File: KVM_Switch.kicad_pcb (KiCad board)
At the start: 6 copper layers, 120 x 120 mm, 77 parts, among them J1 USB_C_Host_B, J2 USB_C_Host_B, J3 Conn_01x02, SW1 SW_Push, U1 TLV62569DBV, U10 USB2514B_M2, U2 AP2112K-3.3, U3 STM32F030C8Tx, U4 TUSB1046A-DCIRNQR, U5 TUSB1046A-DCIRNQR, U6 HD3SS215RTQT, U9 TS3USB221RSERG4, Y1 Crystal

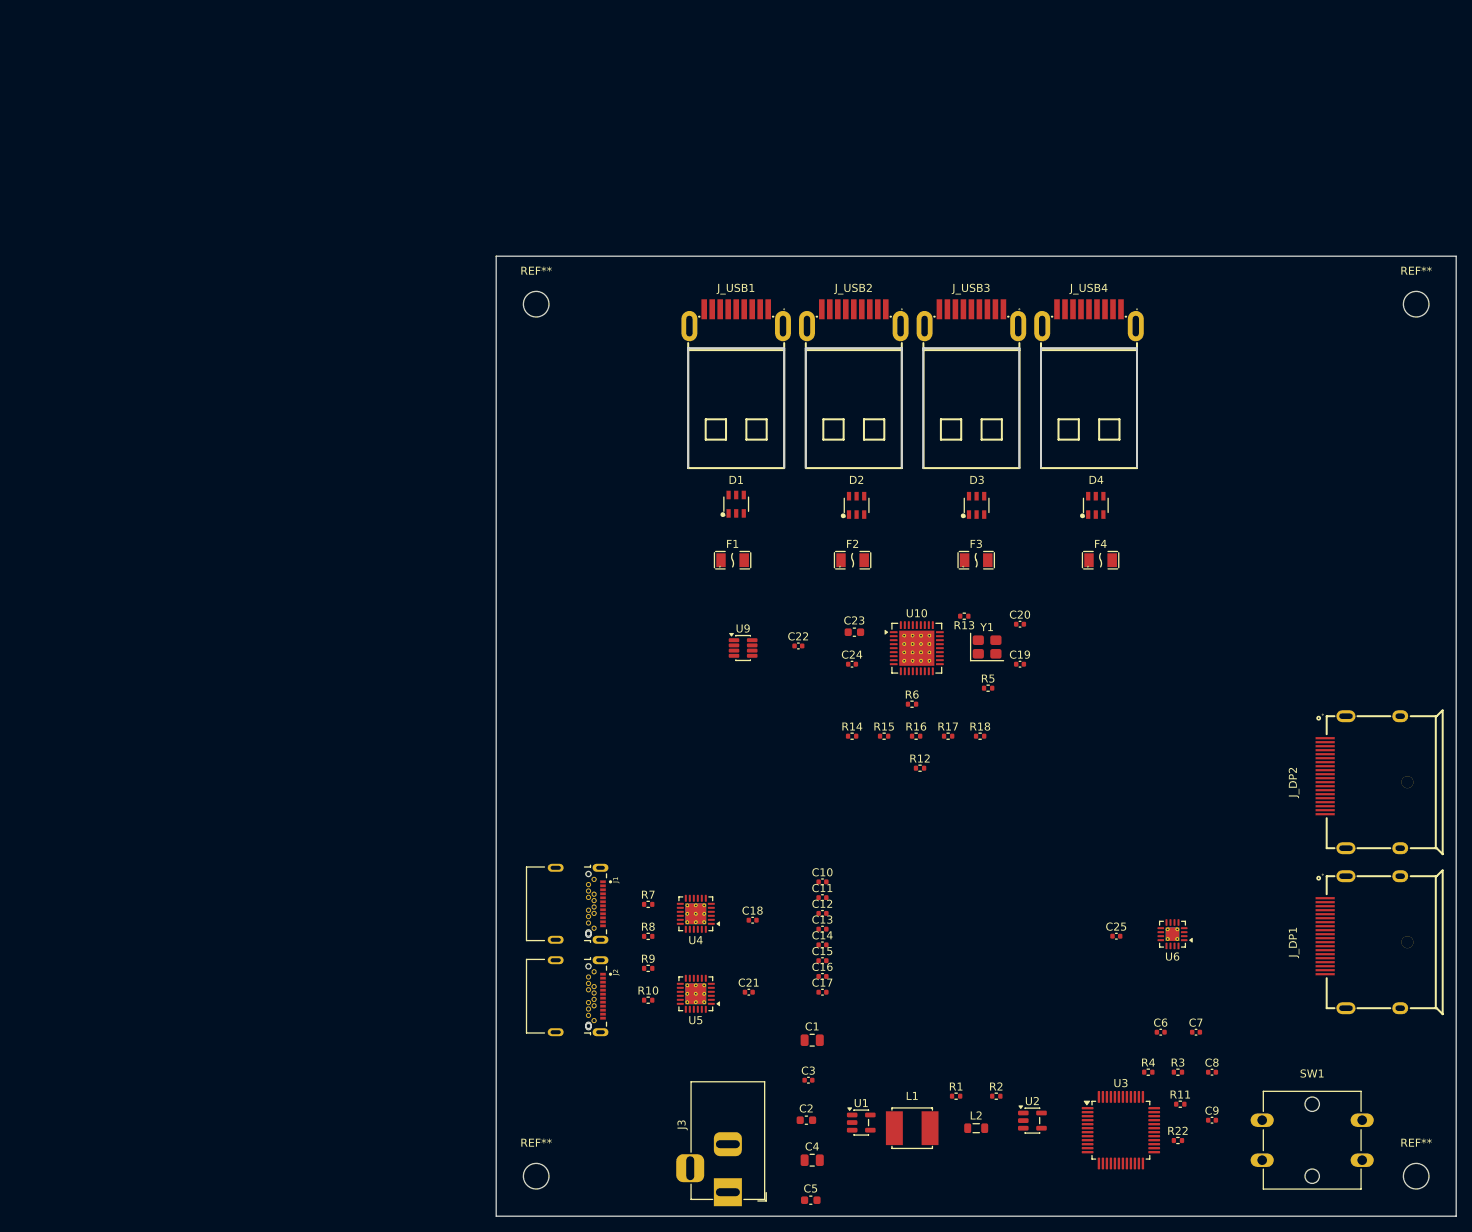
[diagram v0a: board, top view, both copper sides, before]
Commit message: Publish A2 hardware, firmware, and verification package
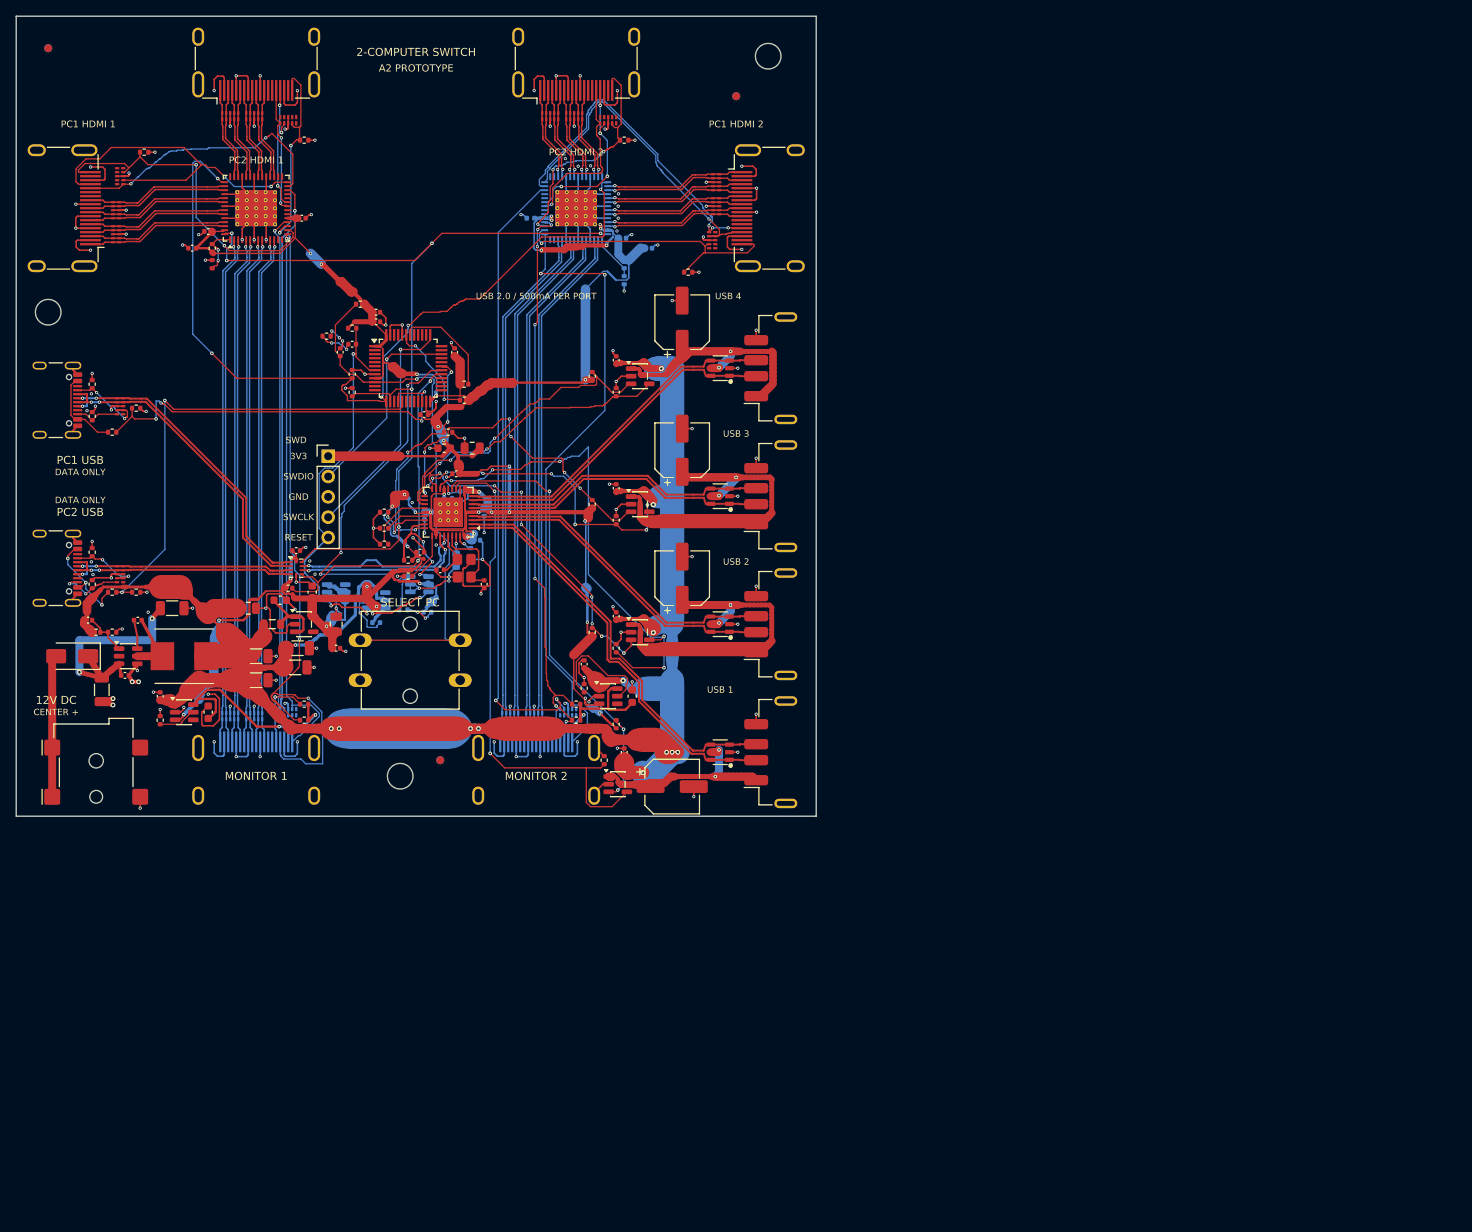
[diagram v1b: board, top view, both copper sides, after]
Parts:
- removed C17: 0.1uF, Capacitor_SMD:C_0402_1005Metric
- removed F1, F2, F3, F4: BSMD1206-050-6V, polyfuse:F1206
- removed J_DP1, J_DP2: 472720001, dp_connector:CONN-SMD_472720001
- removed R5: 1M, Resistor_SMD:R_0402_1005Metric
- removed REF** (x4): MountingHole_3.2mm_M3, MountingHole:MountingHole_3.2mm_M3
- added C26: 1uF, Capacitor_SMD:C_0603_1608Metric, F.Cu at (37.0, 72.0)
- added C27: 100nF, Capacitor_SMD:C_0402_1005Metric, F.Cu at (45.0, 38.2)
- added C28: 100nF, Capacitor_SMD:C_0402_1005Metric, F.Cu at (54.8, 42.0)
- added C29: 100nF, Capacitor_SMD:C_0402_1005Metric, F.Cu at (51.0, 49.8)
- added C30: 10uF, Capacitor_SMD:C_1206_3216Metric, F.Cu at (19.5, 74.0)
- added C31: 100nF, Capacitor_SMD:C_0402_1005Metric, F.Cu at (15.2, 75.5)
- added C32: 1uF, Capacitor_SMD:C_0603_1608Metric, F.Cu at (33.0, 73.0)
- added C33: 150pF, Capacitor_SMD:C_0402_1005Metric, F.Cu at (9.00, 75.5)
- added C34: 100nF, Capacitor_SMD:C_0402_1005Metric, F.Cu at (55.0, 57.2)
- added C35: 100nF, Capacitor_SMD:C_0402_1005Metric, B.Cu at (54.0, 60.3)
- added C36: 100nF, Capacitor_SMD:C_0402_1005Metric, B.Cu at (51.0, 62.4)
- added C37: 100nF, Capacitor_SMD:C_0402_1005Metric, F.Cu at (50.5, 67.0)
- added C38: 100nF, Capacitor_SMD:C_0402_1005Metric, B.Cu at (57.5, 65.5)
- added C39: 100nF, Capacitor_SMD:C_0402_1005Metric, F.Cu at (76.0, 92.0)
- added C40: 100nF, Capacitor_SMD:C_0402_1005Metric, F.Cu at (75.0, 75.0)
- added C41: 100nF, Capacitor_SMD:C_0402_1005Metric, F.Cu at (75.0, 59.0)
- added C42: 100nF, Capacitor_SMD:C_0402_1005Metric, F.Cu at (75.0, 43.0)
- added C43: 220uF, Capacitor_SMD:CP_Elec_6.3x7.7, F.Cu at (82.0, 96.3)
- added C44: 220uF, Capacitor_SMD:CP_Elec_6.3x7.7, F.Cu at (83.2, 70.2)
- added C45: 220uF, Capacitor_SMD:CP_Elec_6.3x7.7, F.Cu at (83.2, 54.2)
- added C46: 220uF, Capacitor_SMD:CP_Elec_6.3x7.7, F.Cu at (83.2, 38.2)
- added C47: 100nF, Capacitor_SMD:C_0402_1005Metric, F.Cu at (18.0, 85.0)
- added C48: 100nF, Capacitor_SMD:C_0402_1005Metric, F.Cu at (71.0, 81.0)
- added C49: 1uF, Capacitor_SMD:C_0603_1608Metric, F.Cu at (24.0, 87.0)
- added C50: 1uF, Capacitor_SMD:C_0603_1608Metric, F.Cu at (77.0, 85.0)
- added C51: 22uF, Capacitor_SMD:C_1206_3216Metric, F.Cu at (34.9, 81.4)
- added C52: 22uF, Capacitor_SMD:C_1206_3216Metric, F.Cu at (35.2, 79.0)
- added C53: 100nF, Capacitor_SMD:C_0402_1005Metric, B.Cu at (40.0, 74.8)
- added C54: 100nF, Capacitor_SMD:C_0402_1005Metric, B.Cu at (45.0, 75.8)
- added C55: 100nF, Capacitor_SMD:C_0402_1005Metric, B.Cu at (51.4, 74.5)
- added D20: SS34, Diode_SMD:D_SMA, F.Cu at (7.00, 80.0)
- added FID1: Fiducial_1mm_Mask2mm, Fiducial_1mm_Mask2mm, F.Cu at (4.00, 4.00)
- added FID2: Fiducial_1mm_Mask2mm, Fiducial_1mm_Mask2mm, F.Cu at (90.0, 10.0)
- added FID3: Fiducial_1mm_Mask2mm, Fiducial_1mm_Mask2mm, F.Cu at (53.0, 93.0)
- added FID4: Fiducial_1mm_Mask2mm, Fiducial_1mm_Mask2mm, B.Cu at (4.00, 4.00)
- added FID5: Fiducial_1mm_Mask2mm, Fiducial_1mm_Mask2mm, B.Cu at (90.0, 10.0)
- added FID6: Fiducial_1mm_Mask2mm, Fiducial_1mm_Mask2mm, B.Cu at (53.0, 93.0)
- added H1: M3 mounting, MountingHole_3.2mm_M3, F.Cu at (4.00, 37.0)
- added H2: M3 mounting, MountingHole_3.2mm_M3, F.Cu at (94.0, 5.00)
- added H3: M3 mounting, MountingHole_3.2mm_M3, F.Cu at (48.0, 95.0)
- added J4: SWD, Connector_PinHeader_2.54mm:PinHeader_1x05_P2.54mm_Vertical, F.Cu at (39.0, 55.0)
- added J_HDMI_C1_MON1: HDMI_A_1.4, KVM_Custom_Footprints:Assembly_J_HDMI_C1_MON1, F.Cu at (6.00, 24.0)
- added J_HDMI_C1_MON2: HDMI_A_1.4, KVM_Custom_Footprints:Assembly_J_HDMI_C1_MON2, F.Cu at (94.0, 24.0)
- added J_HDMI_C2_MON1: HDMI_A_1.4, KVM_Custom_Footprints:Assembly_J_HDMI_C2_MON1, F.Cu at (30.0, 6.00)
- added J_HDMI_C2_MON2: HDMI_A_1.4, KVM_Custom_Footprints:Assembly_J_HDMI_C2_MON2, F.Cu at (70.0, 6.00)
- added J_HDMI_MON1: HDMI_A_1.4, KVM_Custom_Footprints:Assembly_J_HDMI_MON1, B.Cu at (30.0, 94.0)
- added J_HDMI_MON2: HDMI_A_1.4, KVM_Custom_Footprints:Assembly_J_HDMI_MON2, B.Cu at (65.0, 94.0)
- added R19: 100k, Resistor_SMD:R_0402_1005Metric, F.Cu at (84.0, 32.0)
- added R20: 100k, Resistor_SMD:R_0402_1005Metric, F.Cu at (76.0, 15.5)
- added R23: 100k, Resistor_SMD:R_0402_1005Metric, F.Cu at (42.0, 47.0)
- added R24: 100k, Resistor_SMD:R_0402_1005Metric, F.Cu at (42.0, 44.8)
- added R25: 100k, Resistor_SMD:R_0402_1005Metric, F.Cu at (34.0, 71.5)
- added R26: 100k, Resistor_SMD:R_0402_1005Metric, F.Cu at (46.0, 64.0)
- added R27: 100k, Resistor_SMD:R_0402_1005Metric, F.Cu at (46.0, 62.0)
- added R28: 100k, Resistor_SMD:R_0402_1005Metric, F.Cu at (49.0, 70.0)
- added R29: 100k, Resistor_SMD:R_0402_1005Metric, F.Cu at (46.0, 66.0)
- added R30: 100k, Resistor_SMD:R_0402_1005Metric, F.Cu at (73.5, 93.0)
- added R31: 100k, Resistor_SMD:R_0402_1005Metric, F.Cu at (75.0, 79.0)
- added R32: 100k, Resistor_SMD:R_0402_1005Metric, F.Cu at (75.0, 63.0)
- added R33: 100k, Resistor_SMD:R_0402_1005Metric, F.Cu at (75.0, 47.0)
- added R34: 100k, Resistor_SMD:R_0402_1005Metric, F.Cu at (12.0, 52.0)
- added R35: 150k, Resistor_SMD:R_0402_1005Metric, F.Cu at (15.0, 49.0)
- added R36: 100k, Resistor_SMD:R_0402_1005Metric, F.Cu at (12.0, 72.0)
- added R37: 150k, Resistor_SMD:R_0402_1005Metric, F.Cu at (15.0, 72.0)
- added R38: 100k, Resistor_SMD:R_0402_1005Metric, F.Cu at (54.0, 52.0)
- added R39: 10k, Resistor_SMD:R_0402_1005Metric, F.Cu at (75.0, 88.5)
- added R40: 10k, Resistor_SMD:R_0402_1005Metric, F.Cu at (72.0, 77.0)
- added R41: 10k, Resistor_SMD:R_0402_1005Metric, F.Cu at (72.0, 61.0)
- added R42: 10k, Resistor_SMD:R_0402_1005Metric, F.Cu at (72.0, 45.0)
- added R43: 10k, Resistor_SMD:R_0402_1005Metric, F.Cu at (24.5, 29.0)
- added R44: 10k, KVM_Custom_Footprints:Assembly_R44, F.Cu at (24.5, 31.0)
- added R45: 10k, Resistor_SMD:R_0402_1005Metric, B.Cu at (76.0, 31.0)
- added R46: 10k, KVM_Custom_Footprints:Assembly_R46, B.Cu at (76.0, 33.0)
- added R47: 210k, Resistor_SMD:R_0402_1005Metric, F.Cu at (18.0, 88.0)
- added R48: 210k, Resistor_SMD:R_0402_1005Metric, F.Cu at (71.0, 84.0)
- added R49: 10k, Resistor_SMD:R_0402_1005Metric, B.Cu at (48.4, 74.2)
- added R50: 1k, Resistor_SMD:R_0402_1005Metric, F.Cu at (38.8, 40.0)
- added U11: TPD4E02B04DQA, KVM_Custom_Footprints:USON-10_2.5x1.0mm_P0.5mm_Assembly, B.Cu at (64.8, 87.5)
- added U12: TPD4E02B04DQA, KVM_Custom_Footprints:USON-10_2.5x1.0mm_P0.5mm_Assembly, F.Cu at (12.5, 27.2)
- added U13: TPD4E02B04DQA, KVM_Custom_Footprints:USON-10_2.5x1.0mm_P0.5mm_Assembly, F.Cu at (12.5, 24.2)
- added U14: TPD4E02B04DQA, KVM_Custom_Footprints:USON-10_2.5x1.0mm_P0.5mm_Assembly, F.Cu at (26.8, 12.5)
- added U15: TPD4E02B04DQA, KVM_Custom_Footprints:USON-10_2.5x1.0mm_P0.5mm_Assembly, F.Cu at (29.8, 12.5)
- added U16: TPD4E02B04DQA, KVM_Custom_Footprints:USON-10_2.5x1.0mm_P0.5mm_Assembly, F.Cu at (87.5, 20.8)
- added U17: TPD4E02B04DQA, KVM_Custom_Footprints:USON-10_2.5x1.0mm_P0.5mm_Assembly, F.Cu at (87.5, 23.8)
- added U18: TPD4E02B04DQA, KVM_Custom_Footprints:USON-10_2.5x1.0mm_P0.5mm_Assembly, F.Cu at (66.8, 12.5)
- added U19: TPD4E02B04DQA, KVM_Custom_Footprints:USON-10_2.5x1.0mm_P0.5mm_Assembly, F.Cu at (69.8, 12.5)
- added U20: TPS2051CDBVR, Package_TO_SOT_SMD:SOT-23-5, F.Cu at (75.2, 96.0)
- added U21: TPS2051CDBVR, Package_TO_SOT_SMD:SOT-23-5, F.Cu at (78.0, 77.0)
- added U22: TPS2051CDBVR, Package_TO_SOT_SMD:SOT-23-5, F.Cu at (78.0, 61.0)
- added U23: TPS2051CDBVR, Package_TO_SOT_SMD:SOT-23-5, F.Cu at (78.0, 45.0)
- added U24: TPD4E05U06DQAR, KVM_Custom_Footprints:USON-10_2.5x1.0mm_P0.5mm_Assembly, F.Cu at (13.0, 48.8)
- added U25: TPD4E05U06DQAR, KVM_Custom_Footprints:USON-10_2.5x1.0mm_P0.5mm_Assembly, F.Cu at (13.0, 69.8)
- added U26: TPD4E05U06DQAR, KVM_Custom_Footprints:USON-10_2.5x1.0mm_P0.5mm_Assembly, F.Cu at (13.0, 20.0)
- added U27: TPD4E05U06DQAR, KVM_Custom_Footprints:USON-10_2.5x1.0mm_P0.5mm_Assembly, F.Cu at (34.0, 13.0)
- added U28: TPD4E05U06DQAR, KVM_Custom_Footprints:USON-10_2.5x1.0mm_P0.5mm_Assembly, F.Cu at (87.0, 28.0)
- added U29: TPD4E05U06DQAR, KVM_Custom_Footprints:USON-10_2.5x1.0mm_P0.5mm_Assembly, F.Cu at (74.0, 13.0)
- added U30: TPD4E05U06DQAR, KVM_Custom_Footprints:USON-10_2.5x1.0mm_P0.5mm_Assembly, B.Cu at (34.0, 87.0)
- added U31: TPD4E05U06DQAR, KVM_Custom_Footprints:USON-10_2.5x1.0mm_P0.5mm_Assembly, B.Cu at (69.0, 87.0)
- added U32: TPS2553DBVR, Package_TO_SOT_SMD:SOT-23-6, F.Cu at (21.0, 87.0)
- added U33: TPS2553DBVR, Package_TO_SOT_SMD:SOT-23-6, F.Cu at (74.0, 85.0)
- added U34: TPS3808G33DBVR, Package_TO_SOT_SMD:SOT-23-6, B.Cu at (40.0, 72.0)
- added U35: TPS3808G50DBVR, Package_TO_SOT_SMD:SOT-23-6, B.Cu at (45.0, 73.0)
- added U36: SN74LVC1G97DBVR, Package_TO_SOT_SMD:SOT-23-6, B.Cu at (50.4, 71.0)
- added U7: TPD4E02B04DQA, KVM_Custom_Footprints:USON-10_2.5x1.0mm_P0.5mm_Assembly, B.Cu at (61.8, 87.5)
- added U8: HD3SS215IRTQR, Package_DFN_QFN:QFN-56-1EP_8x8mm_P0.5mm_EP4.5x5.2mm_ThermalVias, B.Cu at (70.0, 24.0)
- C1, C4: value 47uF -> 22uF; footprint Capacitor_SMD:C_0805_2012Metric -> Capacitor_SMD:C_1206_3216Metric
- C13, C14, C15, R12: moved to B.Cu
- C16: value 0.1uF -> 10uF; footprint Capacitor_SMD:C_0402_1005Metric -> Capacitor_SMD:C_1206_3216Metric
- C18: value 1uF -> 100nF; footprint Capacitor_SMD:C_0402_1005Metric -> Capacitor_SMD:C_0603_1608Metric; moved to B.Cu
- C19, C20: value 22pF -> 18pF
- C2, C23, C5: footprint Capacitor_SMD:C_0603_1608Metric -> Capacitor_SMD:C_0805_2012Metric
- C21: value 1uF -> 100nF; moved to B.Cu
- C22: value 0.1uF -> 100nF; moved to B.Cu
- C24: footprint Capacitor_SMD:C_0402_1005Metric -> Capacitor_SMD:C_0603_1608Metric
- C25: value 0.1uF -> 100nF
- J1, J2: value USB_C_Host_B -> USB4105-GF-A-120; footprint KVM_Custom_Footprints:CUI_UJ31-CH-G2-SMT-TR -> Connector_USB:USB_C_Receptacle_GCT_USB4105-xx-A_16P_TopMnt_Horizontal
- J3: value Conn_01x02 -> 12V DC center-positive; footprint Connector_BarrelJack:BarrelJack_Horizontal -> Connector_BarrelJack:BarrelJack_Wuerth_694106106102_2.0x5.5mm
- J_USB1: value KH-3.0USB-AM-9P -> USB1046-GF-0190-L-B-A; footprint usb_a_connector:USB-3.0-SMD_KH-3.0USB-AM-9P -> KVM_Custom_Footprints:Assembly_J_USB1
- J_USB2: value KH-3.0USB-AM-9P -> USB1046-GF-0190-L-B-A; footprint usb_a_connector:USB-3.0-SMD_KH-3.0USB-AM-9P -> KVM_Custom_Footprints:Assembly_J_USB2
- J_USB3: value KH-3.0USB-AM-9P -> USB1046-GF-0190-L-B-A; footprint usb_a_connector:USB-3.0-SMD_KH-3.0USB-AM-9P -> KVM_Custom_Footprints:Assembly_J_USB3
- J_USB4: value KH-3.0USB-AM-9P -> USB1046-GF-0190-L-B-A; footprint usb_a_connector:USB-3.0-SMD_KH-3.0USB-AM-9P -> KVM_Custom_Footprints:Assembly_J_USB4
- L1: value 4.7uH -> 6.8uH; footprint inductor_5040:IND-SMD_L5.0-W5.0-1 -> KVM_Custom_Footprints:Bourns_SRP7050TA
- R1: value 750k -> 53.6k
- R14, R15, R16, R6: value 100k -> 47k
- R2: value 100k -> 10k
- U1: value TLV62569DBV -> AP63301WU-7; footprint Package_TO_SOT_SMD:SOT-23-5 -> Package_TO_SOT_SMD:SOT-23-6
- U10: value USB2514B_M2 -> USB2514B-AEZC-TR; footprint Package_DFN_QFN:Texas_RHH0036C_VQFN-36-1EP_6x6mm_P0.5mm_EP4.4x4.4mm_ThermalVias -> Package_DFN_QFN:QFN-36-1EP_6x6mm_P0.5mm_EP3.7x3.7mm_ThermalVias
- U2: value AP2112K-3.3 -> AP2112K-3.3TRG1
- U4, U5: value TUSB1046A-DCIRNQR -> TPD4E02B04DQA; footprint Package_DFN_QFN:WQFN-24-1EP_4x4mm_P0.5mm_EP2.6x2.6mm_ThermalVias -> KVM_Custom_Footprints:USON-10_2.5x1.0mm_P0.5mm_Assembly; moved to B.Cu
- U6: value HD3SS215RTQT -> HD3SS215IRTQR; footprint Package_DFN_QFN:QFN-16-1EP_3x3mm_P0.5mm_EP1.7x1.7mm_ThermalVias -> Package_DFN_QFN:QFN-56-1EP_8x8mm_P0.5mm_EP4.5x5.2mm_ThermalVias
- U9: value TS3USB221RSERG4 -> TS3USB221RSER; footprint Package_TO_SOT_SMD:SOT-23-8 -> Package_DFN_QFN:Texas_UQFN-10_1.5x2mm_P0.5mm
- Y1: value Crystal -> 24MHz 12pF; footprint Crystal:Crystal_SMD_3225-4Pin_3.2x2.5mm -> KVM_Custom_Footprints:Assembly_Y1
- moved U6 146.1 mm to (30.0, 24.0), turned to 90 degrees
- moved C9 145.2 mm to (40.5, 42.0), turned to 90 degrees
- moved C8 140.8 mm to (42.0, 41.0)
- moved R3 138.9 mm to (42.0, 39.0)
- moved R4 137.6 mm to (43.0, 36.0)
- moved C6 133.1 mm to (45.0, 37.0)
- moved U3 130.4 mm to (49.0, 44.0)
- moved R22 128.5 mm to (56.0, 48.0)
- moved SW1 127.7 mm to (43.0, 78.0)
- moved R11 126.9 mm to (56.0, 46.0)
- moved R2 124.8 mm to (12.0, 77.0)
- moved R17 124.2 mm to (16.0, 17.0)
- moved R1 122.1 mm to (10.0, 77.0)
- moved C7 117.7 mm to (40.0, 79.0)
- moved C25 113.3 mm to (35.0, 66.8)
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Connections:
- net Net-(J1-CC1) renamed HOST1_CC1
- net Net-(J1-CC2) renamed HOST1_CC2
- net Net-(J2-CC1) renamed HOST2_CC1
- net Net-(J2-CC2) renamed HOST2_CC2
- net Net-(U10-DM-UP) renamed USB_UP_N
- net Net-(U10-DP-UP) renamed USB_UP_P
- net Net-(U10-~{RESET}) renamed HUB_RESET_N
- net Net-(U2-EN) renamed LDO_VIN
- net Net-(U3-NRST) renamed MCU_NRST
- net USB2_DN_A renamed USB_HOST1_N
- net USB2_DN_B renamed USB_HOST2_N
- net USB2_DP_A renamed USB_HOST1_P
- net USB2_DP_B renamed USB_HOST2_P
- C10 pad 1: Net-(U4-TX2P) -> +3.3V
- C10 pad 2: Net-(U6-DC0(p)) -> GND
- C11 pad 1: Net-(U6-DC0(n)) -> +3.3V
- C11 pad 2: Net-(U4-TX2N) -> GND
- C12 pad 1: Net-(U6-DC2(n)) -> +3.3V
- C12 pad 2: Net-(U4-TX1N) -> GND
- C13 pad 1: Net-(U6-DC2(p)) -> +3.3V
- C13 pad 2: Net-(U4-TX1P) -> GND
- C14 pad 1: Net-(U5-TX2P) -> +3.3V
- C14 pad 2: Net-(U6-DC1(p)) -> GND
- C15 pad 1: Net-(U6-DC1(n)) -> +3.3V
- C15 pad 2: Net-(U5-TX2N) -> GND
- C16 pad 1: Net-(U5-TX1P) -> +VIN
- C16 pad 2: Net-(U6-DC3(p)) -> GND
- C18 pad 1: GND -> HUB_PLLFILT
- C18 pad 2: Net-(U10-PLLFILT) -> GND
- C19 pad 1: GND -> HUB_XTAL1
- C19 pad 2: Net-(U10-XTAL1) -> GND
- C20 pad 1: Net-(U10-XTAL2) -> HUB_XTAL2
- C21 pad 1: GND -> HUB_CRFILT
- C21 pad 2: Net-(U10-CRFILT) -> GND
- C22 pad 1: GND -> +3.3V
- C22 pad 2: +3.3V -> GND
- C23 pad 1: GND -> +3.3V
- C23 pad 2: +3.3V -> GND
- C24 pad 1: GND -> +3.3V
- C24 pad 2: +3.3V -> GND
- C25 pad 1: Net-(U9-VCC) -> +3.3V
- C25 pad 2: +3.3V -> GND
- C3 pad 1: +5V -> +VIN
- C8 pad 1: GND -> RESET_CAP_RETURN
- D1 pad 1: /USB_Hub_ESD/USB_D1_N -> USB_D1_N
- D1 pad 3: /USB_Hub_ESD/USB_D1_P -> USB_D1_P
- D1 pad 4: /USB_Hub_ESD/USB1_DP -> USB_D1_P
- D1 pad 5: +5V -> USB_VBUS1
- D1 pad 6: /USB_Hub_ESD/USB1_DM -> USB_D1_N
- D2 pad 1: /USB_Hub_ESD/USB_D2_N -> USB_D2_N
- D2 pad 3: /USB_Hub_ESD/USB_D2_P -> USB_D2_P
- D2 pad 4: /USB_Hub_ESD/USB2_DP -> USB_D2_P
- D2 pad 5: +5V -> USB_VBUS2
- D2 pad 6: /USB_Hub_ESD/USB2_DM -> USB_D2_N
- D3 pad 1: /USB_Hub_ESD/USB_D3_N -> USB_D3_N
- D3 pad 3: /USB_Hub_ESD/USB_D3_P -> USB_D3_P
- D3 pad 4: /USB_Hub_ESD/USB3_DP -> USB_D3_P
- D3 pad 5: +5V -> USB_VBUS3
- D3 pad 6: /USB_Hub_ESD/USB3_DM -> USB_D3_N
- D4 pad 1: /USB_Hub_ESD/USB_D4_N -> USB_D4_N
- D4 pad 3: /USB_Hub_ESD/USB_D4_P -> USB_D4_P
- D4 pad 4: /USB_Hub_ESD/USB4_DP -> USB_D4_P
- D4 pad 5: +5V -> USB_VBUS4
- D4 pad 6: /USB_Hub_ESD/USB4_DM -> USB_D4_N
- J1 pad A4: unconnected-(J1-VBUS-PadA4)_2 -> HOST1_VBUS
- J1 pad A8: Net-(J1-SBU1) -> unconnected-(J1-SBU1-PadA8)
- J1 pad A9: unconnected-(J1-VBUS-PadA4)_1 -> HOST1_VBUS
- J1 pad B4: unconnected-(J1-VBUS-PadA4) -> HOST1_VBUS
- J1 pad B8: Net-(J1-SBU2) -> unconnected-(J1-SBU2-PadB8)
- J1 pad B9: unconnected-(J1-VBUS-PadA4)_3 -> HOST1_VBUS
- J2 pad A4: unconnected-(J2-VBUS-PadA4)_3 -> HOST2_VBUS
- J2 pad A8: Net-(J2-SBU1) -> unconnected-(J2-SBU1-PadA8)
- J2 pad A9: unconnected-(J2-VBUS-PadA4)_2 -> HOST2_VBUS
- J2 pad B4: unconnected-(J2-VBUS-PadA4) -> HOST2_VBUS
- J2 pad B8: Net-(J2-SBU2) -> unconnected-(J2-SBU2-PadB8)
- J2 pad B9: unconnected-(J2-VBUS-PadA4)_1 -> HOST2_VBUS
- J3 pad 1: /PDN/+VIN -> VIN_RAW
- J_USB1 pad 1: /USB_Hub_ESD/USB1_VBUS -> USB_VBUS1
- J_USB1 pad 2: /USB_Hub_ESD/USB1_DM -> USB_D1_N
- J_USB1 pad 3: /USB_Hub_ESD/USB1_DP -> USB_D1_P
- J_USB2 pad 1: /USB_Hub_ESD/USB2_VBUS -> USB_VBUS2
- J_USB2 pad 2: /USB_Hub_ESD/USB2_DM -> USB_D2_N
- J_USB2 pad 3: /USB_Hub_ESD/USB2_DP -> USB_D2_P
- J_USB3 pad 1: /USB_Hub_ESD/USB3_VBUS -> USB_VBUS3
- J_USB3 pad 2: /USB_Hub_ESD/USB3_DM -> USB_D3_N
- J_USB3 pad 3: /USB_Hub_ESD/USB3_DP -> USB_D3_P
- J_USB4 pad 1: /USB_Hub_ESD/USB4_VBUS -> USB_VBUS4
- J_USB4 pad 2: /USB_Hub_ESD/USB4_DM -> USB_D4_N
- J_USB4 pad 3: /USB_Hub_ESD/USB4_DP -> USB_D4_P
- L1 pad 1: Net-(U1-SW) -> BUCK_SW
- R1 pad 1: Net-(U1-FB) -> +5V
- R1 pad 2: +5V -> BUCK_FB
- R12 pad 1: GND -> HUB_RBIAS
- R12 pad 2: Net-(U10-RBIAS) -> GND
- R14 pad 1: GND -> /USBC_Mux/MON1_DDC_DAT
- R14 pad 2: Net-(J_DP1-Pad14) -> HDMI_MON1_5V
- R15 pad 1: /USBC_Mux/HPDA -> /USBC_Mux/MON2_DDC_CLK
- R15 pad 2: GND -> HDMI_MON2_5V
- R16 pad 1: GND -> /USBC_Mux/MON2_DDC_DAT
- R16 pad 2: Net-(J_DP2-Pad14) -> HDMI_MON2_5V
- R17 pad 1: /USBC_Mux/HPDB -> /USBC_Mux/C1_MON1_HPD
- R18 pad 1: GND -> /USBC_Mux/C2_MON1_HPD
- R18 pad 2: Net-(J_DP2-Pad13) -> GND
- R2 pad 1: Net-(U1-FB) -> BUCK_FB
- R6 pad 1: GND -> /USBC_Mux/MON1_DDC_CLK
- R6 pad 2: Net-(J_DP1-Pad13) -> HDMI_MON1_5V
- U1 pad 1: /PDN/+VIN -> BUCK_FB
- U1 pad 2: GND -> unconnected-(U1-EN-Pad2)
- U1 pad 3: Net-(U1-SW) -> +VIN
- U1 pad 4: /PDN/+VIN -> GND
- U1 pad 5: Net-(U1-FB) -> BUCK_SW
- U10 pad 1: /USB_Hub_ESD/USB_D1_N -> USB_D1_N
- U10 pad 12: unconnected-(U10-PRTPWR1-Pad12) -> USB_PWR1
- U10 pad 13: unconnected-(U10-OCS1-Pad13) -> USB_OC1_N
- U10 pad 14: Net-(U10-CRFILT) -> HUB_CRFILT
- U10 pad 16: unconnected-(U10-PRTPWR2-Pad16) -> USB_PWR2
- U10 pad 17: unconnected-(U10-OCS2-Pad17) -> USB_OC2_N
- U10 pad 18: unconnected-(U10-PRTPWR3-Pad18) -> USB_PWR3
- U10 pad 19: unconnected-(U10-OCS3-Pad19) -> USB_OC3_N
- U10 pad 2: /USB_Hub_ESD/USB_D1_P -> USB_D1_P
- U10 pad 20: unconnected-(U10-PRTPWR4-Pad20) -> USB_PWR4
- U10 pad 21: unconnected-(U10-OCS4-Pad21) -> USB_OC4_N
- U10 pad 22: unconnected-(U10-SMBDATA-Pad22) -> HUB_NONREM1
- U10 pad 24: unconnected-(U10-SMBCLK-Pad24) -> HUB_CFG0
- U10 pad 25: GND -> HUB_CFG1
- U10 pad 27: +3.3V -> HUB_VBUS_DET
- U10 pad 28: unconnected-(U10-SUSP_IND-Pad28) -> HUB_NONREM0
- U10 pad 3: /USB_Hub_ESD/USB_D2_N -> USB_D2_N
- U10 pad 32: Net-(U10-XTAL1) -> HUB_XTAL1
- U10 pad 33: Net-(U10-XTAL2) -> HUB_XTAL2
- U10 pad 34: Net-(U10-PLLFILT) -> HUB_PLLFILT
- U10 pad 35: Net-(U10-RBIAS) -> HUB_RBIAS
- U10 pad 4: /USB_Hub_ESD/USB_D2_P -> USB_D2_P
- U10 pad 6: /USB_Hub_ESD/USB_D3_N -> USB_D3_N
- U10 pad 7: /USB_Hub_ESD/USB_D3_P -> USB_D3_P
- U10 pad 8: /USB_Hub_ESD/USB_D4_N -> USB_D4_N
- U10 pad 9: /USB_Hub_ESD/USB_D4_P -> USB_D4_P
- U3 pad 11: TUSB2_SEL -> unconnected-(U3-PA1-Pad11)
- U3 pad 12: TUSB1_SEL -> unconnected-(U3-PA2-Pad12)
- U3 pad 16: unconnected-(U3-PA6-Pad16) -> HOST1_PRESENT
- U3 pad 17: unconnected-(U3-PA7-Pad17) -> HOST2_PRESENT
- U3 pad 29: unconnected-(U3-PA8-Pad29) -> USB_OE_N
- U3 pad 30: unconnected-(U3-PA9-Pad30) -> HUB_RESET_REQ
- U3 pad 31: unconnected-(U3-PA10-Pad31) -> HUB_VBUS_DET
- U3 pad 34: unconnected-(U3-PA13-Pad34) -> SWDIO
- U3 pad 37: unconnected-(U3-PA14-Pad37) -> SWCLK
- U4 pad 1: +3.3V -> /USBC_Mux/MON1_D2_P
- U4 pad 10: Net-(J1-TX2+) -> /USBC_Mux/MON1_D2_P
- U4 pad 2: unconnected-(U4-DPEQ1-Pad2) -> /USBC_Mux/MON1_D2_N
- U4 pad 3: unconnected-(U4-SSEQ1-Pad3) -> GND
- U4 pad 4: Net-(J1-TX1+) -> /USBC_Mux/MON1_D1_P
- U4 pad 5: Net-(J1-TX1-) -> /USBC_Mux/MON1_D1_N
- U4 pad 6: +3.3V -> /USBC_Mux/MON1_D1_N
- U4 pad 7: Net-(J1-RX1+) -> /USBC_Mux/MON1_D1_P
- U4 pad 8: Net-(J1-RX1-) -> GND
- U4 pad 9: Net-(J1-TX2-) -> /USBC_Mux/MON1_D2_N
- U5 pad 1: +3.3V -> /USBC_Mux/MON1_D0_P
- U5 pad 10: Net-(J2-TX2+) -> /USBC_Mux/MON1_D0_P
- U5 pad 2: unconnected-(U5-DPEQ1-Pad2) -> /USBC_Mux/MON1_D0_N
- U5 pad 3: unconnected-(U5-SSEQ1-Pad3) -> GND
- U5 pad 4: Net-(J2-TX1+) -> /USBC_Mux/MON1_D3_P
- U5 pad 5: Net-(J2-TX1-) -> /USBC_Mux/MON1_D3_N
- U5 pad 6: +3.3V -> /USBC_Mux/MON1_D3_N
- U5 pad 7: Net-(J2-RX1+) -> /USBC_Mux/MON1_D3_P
- U5 pad 8: Net-(J2-RX1-) -> GND
- U5 pad 9: Net-(J2-TX2-) -> /USBC_Mux/MON1_D0_N
- U6 pad 1: unconnected-(U6-AUX_SEL-Pad1) -> HDMI_MODE_1
- U6 pad 11: Net-(U6-DC3(p)) -> /USBC_Mux/MON1_D3_P
- U6 pad 12: Net-(U6-DC3(n)) -> /USBC_Mux/MON1_D3_N
- U6 pad 15: unconnected-(U6-HPDC-Pad15) -> /USBC_Mux/MON1_HPD
- U6 pad 16: /USBC_Mux/HPDA -> /USBC_Mux/C1_MON1_HPD
- U6 pad 17: /USBC_Mux/HPDB -> /USBC_Mux/C2_MON1_HPD
- U6 pad 2: Net-(U6-DC0(p)) -> /USBC_Mux/MON1_D2_P
- U6 pad 3: Net-(U6-DC0(n)) -> /USBC_Mux/MON1_D2_N
- U6 pad 5: Net-(U6-DC1(p)) -> /USBC_Mux/MON1_D1_P
- U6 pad 6: Net-(U6-DC1(n)) -> /USBC_Mux/MON1_D1_N
- U6 pad 8: Net-(U6-DC2(p)) -> /USBC_Mux/MON1_D0_P
- U6 pad 9: Net-(U6-DC2(n)) -> /USBC_Mux/MON1_D0_N
- U9 pad 6: GND -> USB_OE_N
- Y1 pad 1: Net-(U10-XTAL1) -> HUB_XTAL1
- Y1 pad 2: Net-(U10-XTAL2) -> GND
- Y1 pad 3: (no net) -> HUB_XTAL2
- Y1 pad 4: (no net) -> GND
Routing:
- net +3.3V: track 0.00 -> 405.5 mm, vias 0 -> 38
- net GND: track 0.00 -> 390.8 mm, vias 0 -> 149
- net +5V: track 0.00 -> 264.2 mm, vias 0 -> 13
- net /USBC_Mux/MON1_DDC_DAT: track 0.00 -> 213.7 mm, vias 0 -> 3
- net HOST_SELECT: track 0.00 -> 114.6 mm, vias 0 -> 6
- net MUX_RESET: track 0.00 -> 105.4 mm, vias 0 -> 5
- net /USBC_Mux/MON2_DDC_DAT: track 0.00 -> 84.0 mm, vias 0 -> 3
- net /USBC_Mux/MON2_HPD: track 0.00 -> 78.9 mm, vias 0 -> 2
- net /USBC_Mux/MON1_DDC_CLK: track 0.00 -> 71.9 mm, vias 0 -> 2
- net /USBC_Mux/MON2_DDC_CLK: track 0.00 -> 71.4 mm, vias 0 -> 6
- net Net-(U3-PA0): track 0.00 -> 69.9 mm, vias 0 -> 1
- net /USBC_Mux/MON1_HPD: track 0.00 -> 68.6 mm, vias 0 -> 1
- net /USBC_Mux/MON2_D3_N: track 0.00 -> 65.8 mm
- net /USBC_Mux/MON2_D0_N: track 0.00 -> 65.8 mm
- net /USBC_Mux/MON2_D1_P: track 0.00 -> 65.8 mm
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- added copper zone on In1.Cu, net GND
- added copper zone on In2.Cu, net GND
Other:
- board size 120 x 120 mm -> 100 x 100 mm
- copper layers 6 -> 4
- board text added: "12V DC"
- board text added: "2-COMPUTER SWITCH"
- board text added: "3V3"
- board text added: "A2 PROTOTYPE"
- board text added: "CENTER +"
- board text added: "DATA ONLY"
- board text added: "GND"
- board text added: "MONITOR 1"
- board text added: "MONITOR 2"
- board text added: "PC1 HDMI 1"
- board text added: "PC1 HDMI 2"
- board text added: "PC1 USB"
- board text added: "PC2 HDMI 1"
- board text added: "PC2 HDMI 2"
- board text added: "PC2 USB"
- board text added: "RESET"
- board text added: "SELECT PC"
- board text added: "SWCLK"
- board text added: "SWD"
- board text added: "SWDIO"
- board text added: "USB 1"
- board text added: "USB 2"
- board text added: "USB 2.0 / 500mA PER PORT"
- board text added: "USB 3"
- board text added: "USB 4"
